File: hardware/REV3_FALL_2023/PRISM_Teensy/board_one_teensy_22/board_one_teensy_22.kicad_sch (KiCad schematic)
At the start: 21 parts, among them J1 DM3CS-SF, J2 PRISM_IO_INTERFACE, J3 3387, U1 Teensy4.0, U2 GPS-14414, U3 3966, U4 RFM69HCW_Breakout

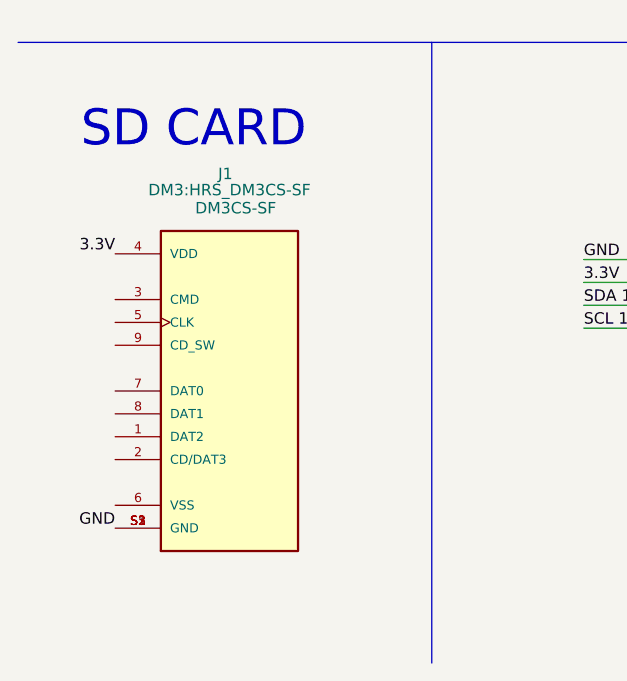
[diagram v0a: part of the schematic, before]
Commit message: Added Parts
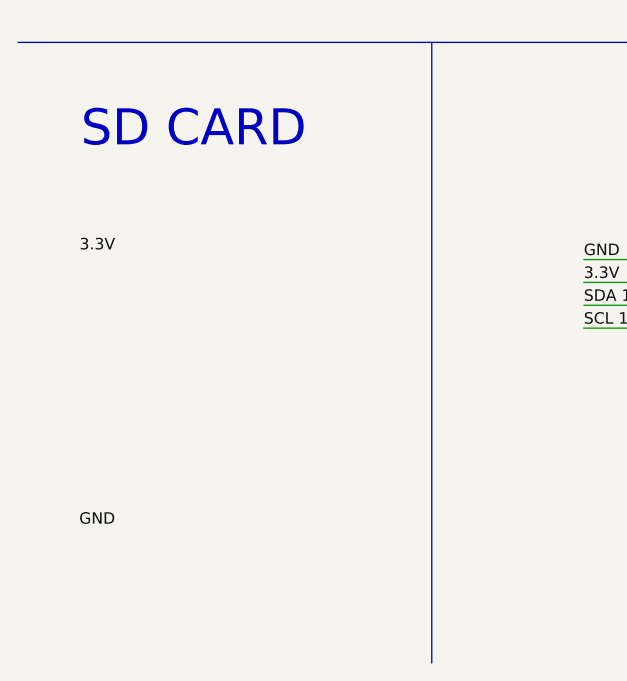
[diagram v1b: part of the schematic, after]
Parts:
- removed J1: DM3CS-SF, DM3:HRS_DM3CS-SF, symbol DM3:DM3CS-SF
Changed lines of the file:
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@@
-    )
-  )
-  (symbol (lib_id "DM3:DM3CS-SF") (at 35.56 167.64 0) (unit 1)
-    (in_bom yes) (on_board yes) (dnp no)
-    (property "Reference" "J1" (at 34.29 143.51 0)
-      (effects (font (size 1.27 1.27)) (justify left))
-    )
-    (property "Value" "DM3CS-SF" (at 31.75 147.32 0)
-      (effects (font (size 1.27 1.27)) (justify left))
-    )
-    (property "Footprint" "DM3:HRS_DM3CS-SF" (at 35.56 146.05 0)
-      (effects (font (size 1.27 1.27)) (justify bottom))
-    )
-    (property "Datasheet" "" (at 35.56 167.64 0)
-      (effects (font (size 1.27 1.27)) hide)
-    )
-    (property "MF" "Hirose" (at 35.56 167.64 0)
-      (effects (font (size 1.27 1.27)) (justify bottom) hide)
-    )
-    (property "DESCRIPTION" "CONN MICRO SD CARD HINGED TYPE" (at 35.56 167.64 0)
-      (effects (font (size 1.27 1.27)) (justify bottom) hide)
-    )
-    (property "PACKAGE" "None" (at 35.56 167.64 0)
-      (effects (font (size 1.27 1.27)) (justify bottom) hide)
-    )
-    (property "PRICE" "1.14 USD" (at 35.56 167.64 0)
-      (effects (font (size 1.27 1.27)) (justify bottom) hide)
-    )
-    (property "Package" "None" (at 35.56 167.64 0)
-      (effects (font (size 1.27 1.27)) (justify bottom) hide)
-    )
-    (property "Check_prices" "https://www.snapeda.com/parts/DM3CS-SF/Hirose+Electric+Co+Ltd/view-part/?ref=eda" (at 35.56 167.64 0)
-      (effects (font (size 1.27 1.27)) (justify bottom) hide)
-    )
-    (property "Availability" "In Stock" (at 35.56 167.64 0)
-      (effects (font (size 1.27 1.27)) (justify bottom) hide)
-    )
-    (property "Price" "None" (at 35.56 167.64 0)
-      (effects (font (size 1.27 1.27)) (justify bottom) hide)
-    )
-    (property "PARTREV" "n/a" (at 35.56 167.64 0)
-      (effects (font (size 1.27 1.27)) (justify bottom) hide)
-    )
-    (property "SnapEDA_Link" "https://www.snapeda.com/parts/DM3CS-SF/Hirose+Electric+Co+Ltd/view-part/?ref=snap" (at 35.56 167.64 0)
-      (effects (font (size 1.27 1.27)) (justify bottom) hide)
-    )
-    (property "MP" "DM3CS-SF" (at 35.56 167.64 0)
-      (effects (font (size 1.27 1.27)) (justify bottom) hide)
-    )
-    (property "Purchase-URL" "https://www.snapeda.com/api/url_track_click_mouser/?unipart_id=189585&manufacturer=Hirose&part_name=DM3CS-SF&search_term=dm3cs-sf" (at 35.56 167.64 0)
-      (effects (font (size 1.27 1.27)) (justify bottom) hide)
-    )
-    (property "Description" "\n10 (8 + 2) Position Card Connector Secure Digital - microSD™ Surface Mount, Right Angle Gold\n" (at 35.56 167.64 0)
-      (effects (font (size 1.27 1.27)) (justify bottom) hide)
-    )
-    (property "STANDARED" "manufacturer recommendation" (at 35.56 167.64 0)
-      (effects (font (size 1.27 1.27)) (justify bottom) hide)
-    )
-    (property "AVAILABILITY" "Good" (at 35.56 167.64 0)
-      (effects (font (size 1.27 1.27)) (justify bottom) hide)
-    )
-    (property "MANUFACTURER" "Hirose" (at 35.56 167.64 0)
-      (effects (font (size 1.27 1.27)) (justify bottom) hide)
-    )
-    (pin "1")
-    (pin "2")
-    (pin "3")
-    (pin "4")
-    (pin "5")
-    (pin "6")
-    (pin "7")
-    (pin "8")
-    (pin "9")
-    (pin "S1")
-    (pin "S2")
-    (pin "S3")
-    (pin "S5")
-    (instances
-      (project "board_one_teensy_22"
-        (path "/7a48c3b0-2761-409e-ae2f-7ebae3820225"
-          (reference "J1") (unit 1)
-        )
-      )
     )
   )
